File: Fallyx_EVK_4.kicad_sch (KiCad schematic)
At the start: 0 parts

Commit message: continued design work
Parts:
- added C10, C17, C18, C24, C25: 10pF, Capacitor_SMD:C_0402_1005Metric, symbol Device:C
- added C11, C13, C23: 1uF, Capacitor_SMD:C_0402_1005Metric, symbol Device:C
- added C12, C15, C16, C19, C20, C21, C22, C26: 0.1uF, Capacitor_SMD:C_0402_1005Metric, symbol Device:C
- added C14: 4.7uF, Capacitor_SMD:C_0603_1608Metric, symbol Device:C
- added C9: 22nuF, Capacitor_SMD:C_0402_1005Metric, symbol Device:C
- added FB1: 600R/0.7A, symbol Device:FerriteBead
- added R11, R14: 10k, Resistor_SMD:R_0402_1005Metric, symbol Device:R_US
- added R12: 1k, Resistor_SMD:R_0402_1005Metric, symbol Device:R_US
- added R13: 0R, Resistor_SMD:R_0805_2012Metric, symbol Device:R_US
- added U4: STM32L431VCIx, Package_BGA:UFBGA-100_7x7mm_Layout12x12_P0.5mm, symbol MCU_ST_STM32L4:STM32L431VCIx
- added U5: MX25R3235FZNxx0, Package_SON:WSON-8-1EP_6x5mm_P1.27mm_EP3.4x4mm, symbol Memory_Flash:MX25R3235FZNxx0
- added X1: 8MHz, ECS-320-CDX-2094:XTAL_ECS-320-CDX-2094, symbol Device:Crystal
- added X2: 32.768kHz, CM9V-T1A-32.768KHZ-7PF-100PPM-TA-QC:XTAL_CM9V-T1A-32.768KHZ-7PF-100PPM-TA-QC, symbol Device:Crystal
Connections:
- new net: C10.1, R12.2, U4.H2 (NRST)
- new net 1V8: C14.1, C15.1, C16.1, C19.1, C20.1, C21.1, C22.1, FB1.2, R14.2, U4.C11 (VDD), U4.C4 (VDD), U4.G11 (VDD), U4.G12 (VDD), U4.G2 (VDD), U4.H3 (VDD), U5.8 (VCC)
- new net BLE_UART_RX: U4.A6 (PD5)
- new net BLE_UART_TX: U4.B6 (PD6)
- new net ENHV: U4.D12 (PC9)
- new net ENLV: U4.B11 (PC10)
- new net GND: C10.2, C11.2, C12.2, C13.2, C14.2, C15.2, C16.2, C17.2, C18.2, C19.2, C20.2, C21.2, C22.2, C23.2, C24.2, C25.2, C26.2, C9.2, R11.1, U4.D3 (VSS), U4.E3 (VSS), U4.F11 (VSS), U4.F12 (VSS), U4.F2 (VSS), U4.J1 (VSSA), U4.K1 (VREF-), U5.4 (GND), U5.9 (GND)
- new net GPOUT: U4.J3 (PC2)
- new net I2C1_SCL: U4.A3 (PB8)
- new net I2C1_SDA: U4.B3 (PB9)
- new net I2C2_SCL: U4.L10 (PB10)
- new net I2C2_SDA: U4.L11 (PB11)
- new net JTMS_SWCLK: U4.A10 (PA14)
- new net JTMS_SWDIO: U4.A11 (PA13)
- new net MCP_STAT: U4.B7 (PD4)
- new net NRF_nRESET: U4.B1 (PE4)
- new net PA0: U4.L2 (PA0)
- new net PA1: U4.M2 (PA1)
- new net PA10: U4.C12 (PA10)
- new net PA9: U4.D10 (PA9)
- new net PB0: U4.M5 (PB0)
- new net PB1: U4.M6 (PB1)
- new net PB12: U4.L12 (PB12)
- new net PB13: U4.K12 (PB13)
- new net PC0: U4.H1 (PC0)
- new net PC1: U4.J2 (PC1)
- new net PC4: U4.K5 (PC4)
- new net PC5: U4.L5 (PC5)
- new net PC6: U4.E12 (PC6)
- new net PD7: U4.A5 (PD7)
- new net PE3: U4.A1 (PE3)
- new net PE6: U4.D2 (PE6)
- new net PE7: U4.M7 (PE7)
- new net PE9: U4.M8 (PE9)
- new net QSPI_BK1_CLK: U4.L8 (PE10), U5.6 (SCLK)
- new net QSPI_BK1_IO0: U4.L9 (PE12), U5.5 (SI/SIO0)
- new net QSPI_BK1_IO1: U4.M10 (PE13), U5.2 (SO/SIO1)
- new net QSPI_BK1_IO2: U4.M11 (PE14), U5.3 (~{WP}/SIO2)
- new net QSPI_BK1_IO3: U4.M12 (PE15), U5.7 (~{RESET}/SIO3)
- new net QSPI_BK1_NCS: R14.1, U4.M9 (PE11), U5.1 (~{CS})
- new net SINK1: U4.K8 (PD9)
- new net SPI1_MISO: U4.L4 (PA6)
- new net SPI1_MOSI: U4.M4 (PA7)
- new net SPI1_SCK: U4.K4 (PA5)
- new net SPI_LEVEL_EN: U4.B8 (PD3)
- new net STM_BOOT0: R11.2, U4.A4 (PH3)
- new net STM_HS_N: C17.1, U4.F1 (PH0), X1.2
- new net STM_HS_P: C18.1, U4.G1 (PH1), X1.1
- new net STM_RTC_N: C24.1, U4.D1 (PC14), X2.2
- new net STM_RTC_P: C25.1, U4.E1 (PC15), X2.1
- new net STM_STATUS0: U4.K9 (PD8)
- new net STM_STATUS1: U4.J11 (PD11)
- new net STM_STATUS2: U4.J12 (PD10)
- new net STM_VDDA: C12.1, C13.1, C23.1, C26.1, FB1.1, U4.L1 (VREF+), U4.M1 (VDDA)
- new net STM_nRST: C9.1, R12.1
- new net VBAT: C11.1, R13.2, U4.E2 (VBAT)
- new net VRTC: R13.1
- no-connect marks 0 -> 32
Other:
- note added: "HIGH FREQ CLK"
- note added: "LOW FREQ CLK"
- note added: "MX25R6435FZNIL0"
- note added: "SPI FLASH"
- note added: "STM32 CONTROLLER"

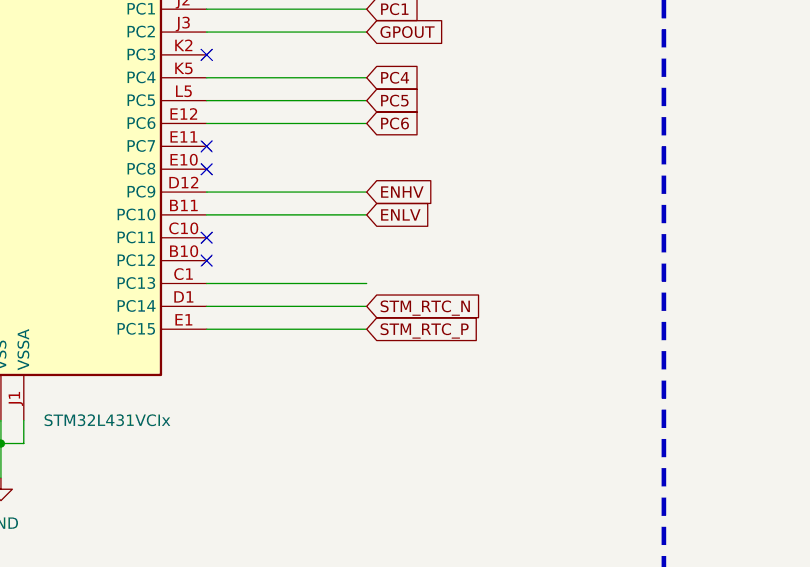
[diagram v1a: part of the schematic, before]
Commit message: review edits
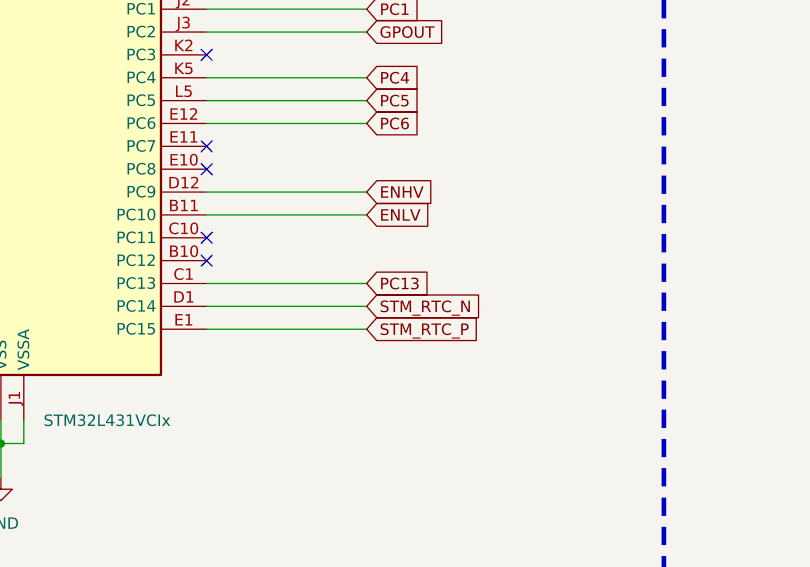
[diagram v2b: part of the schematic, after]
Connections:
- net PC13: now reaches U4.C1 (PC13)
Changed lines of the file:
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@@
+		)
+	)
+	(global_label "PC13"
+		(shape input)
+		(at 133.35 162.56 0)
+		(fields_autoplaced yes)
+		(effects
+			(font
+				(size 1.27 1.27)
+				(color 0 60 135 1)
+			)
+			(justify left)
+		)
+		(property "Intersheetrefs" "${INTERSHEET_REFS}"
+			(at 141.2942 162.56 0)
+			(effects
+				(font
+					(size 1.27 1.27)
+				)
+				(justify left)
+				(hide yes)
+			)
 		)
 	)
